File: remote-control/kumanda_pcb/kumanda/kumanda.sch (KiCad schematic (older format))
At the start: 37 parts, among them J1 USB_A, J2 Conn_01x04, J3 RJ45, J4 Conn_01x06, J5 Screw_Terminal_01x02, U1 MEGA_PRO_EMBED_CH340G___ATMEG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

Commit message: Schematic finished
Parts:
- AV1, CAN_H1, CAN_L1: footprint (none) -> Connector_PinHeader_2.54mm:PinHeader_1x01_P2.54mm_Vertical
- J5: footprint (none) -> TerminalBlock_Phoenix:TerminalBlock_Phoenix_PT-1,5-2-3.5-H_1x02_P3.50mm_Horizontal
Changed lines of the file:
@@
 F 0 "AV1" V 4414 6512 50  0000 R CNN
 F 1 "Conn_01x01" V 4323 6512 50  0000 R CNN
-F 2 "" H 4450 6600 50  0001 C CNN
+F 2 "Connector_PinHeader_2.54mm:PinHeader_1x01_P2.54mm_Vertical" H 4450 6600 50  0001 C CNN
 F 3 "~" H 4450 6600 50  0001 C CNN
 	1    4450 6600
@@
 F 0 "CAN_L1" V 5714 6512 50  0000 R CNN
 F 1 "Conn_01x01" V 5623 6512 50  0000 R CNN
-F 2 "" H 5750 6600 50  0001 C CNN
+F 2 "Connector_PinHeader_2.54mm:PinHeader_1x01_P2.54mm_Vertical" H 5750 6600 50  0001 C CNN
 F 3 "~" H 5750 6600 50  0001 C CNN
 	1    5750 6600
@@
 F 0 "CAN_H1" V 5214 6462 50  0000 R CNN
 F 1 "Conn_01x01" V 5123 6462 50  0000 R CNN
-F 2 "" H 5250 6550 50  0001 C CNN
+F 2 "Connector_PinHeader_2.54mm:PinHeader_1x01_P2.54mm_Vertical" H 5250 6550 50  0001 C CNN
 F 3 "~" H 5250 6550 50  0001 C CNN
 	1    5250 6550
@@
 F 0 "J5" H 1043 3450 50  0000 C CNN
 F 1 "Screw_Terminal_01x02" H 1043 3541 50  0000 C CNN
-F 2 "" H 1125 3775 50  0001 C CNN
+F 2 "TerminalBlock_Phoenix:TerminalBlock_Phoenix_PT-1,5-2-3.5-H_1x02_P3.50mm_Horizontal" H 1125 3775 50  0001 C CNN
 F 3 "~" H 1125 3775 50  0001 C CNN
 	1    1125 3775

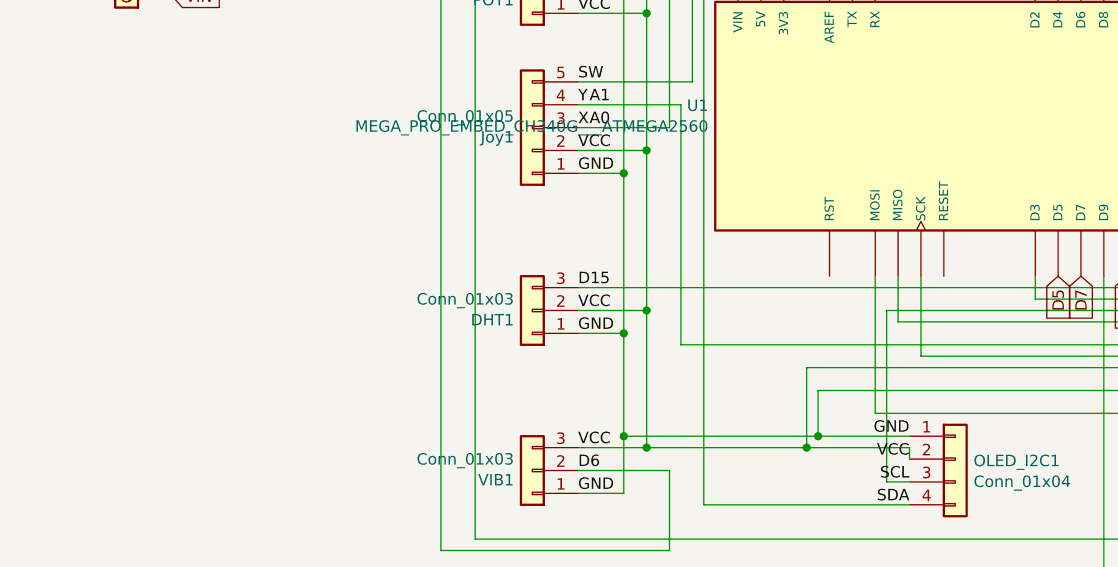
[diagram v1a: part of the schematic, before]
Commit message: Schematic finished.
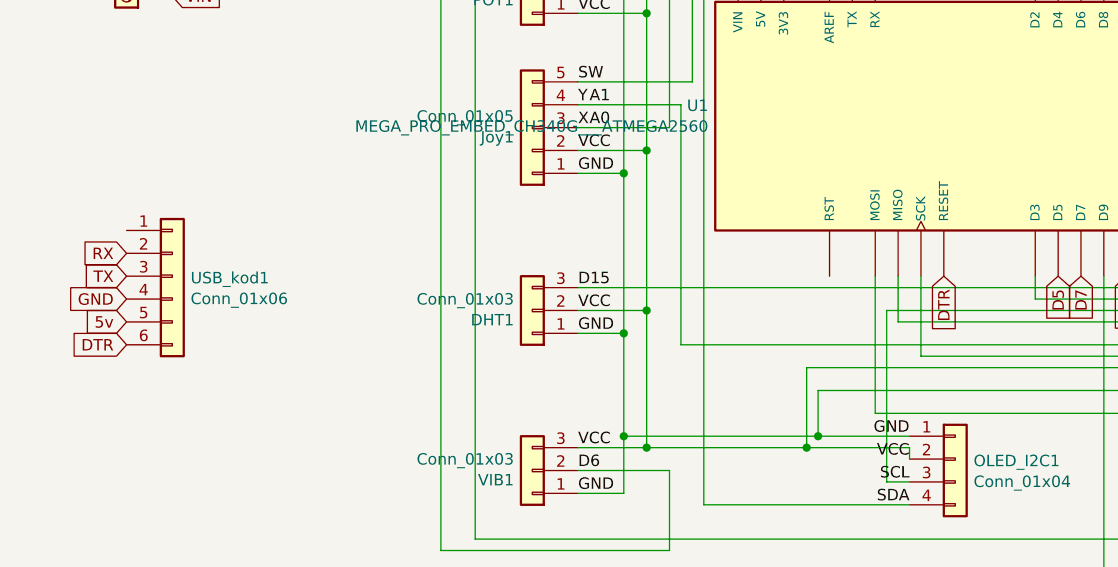
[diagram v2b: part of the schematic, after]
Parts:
- added USB_kod1: Conn_01x06, Connector_PinHeader_2.54mm:PinHeader_1x06_P2.54mm_Vertical, symbol Connector_Generic:Conn_01x06
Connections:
- net GND: now also USB_kod1.4 (Pin_4)
- net RX: now also USB_kod1.2 (Pin_2)
- net TX: now also USB_kod1.3 (Pin_3)
- net DTR: now reaches U1.RESET
- net DTR: now also USB_kod1.6 (Pin_6)
- new net 5v: USB_kod1.5 (Pin_5)
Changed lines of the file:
@@
 Text GLabel 3800 3600 1    50   Input ~ 0
 VIN
+$Comp
+L Connector_Generic:Conn_01x06 USB_kod1
+U 1 1 60CFD659
+P 1325 5000
+F 0 "USB_kod1" H 1405 4992 50  0000 L CNN
+F 1 "Conn_01x06" H 1405 4901 50  0000 L CNN
+F 2 "Connector_PinHeader_2.54mm:PinHeader_1x06_P2.54mm_Vertical" H 1325 5000 50  0001 C CNN
+F 3 "~" H 1325 5000 50  0001 C CNN
+	1    1325 5000
+	1    0    0    -1
+$EndComp
+Text GLabel 1125 4900 0    50   Input ~ 0
+RX
+Text GLabel 1125 5000 0    50   Input ~ 0
+TX
+Text GLabel 1125 5100 0    50   Input ~ 0
+GND
+Text GLabel 1125 5200 0    50   Input ~ 0
+5v
+Text GLabel 1125 5300 0    50   Input ~ 0
+DTR
+Text GLabel 4700 5000 3    50   Input ~ 0
+DTR
 $EndSCHEMATC
